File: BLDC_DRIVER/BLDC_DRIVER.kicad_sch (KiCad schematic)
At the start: 0 parts

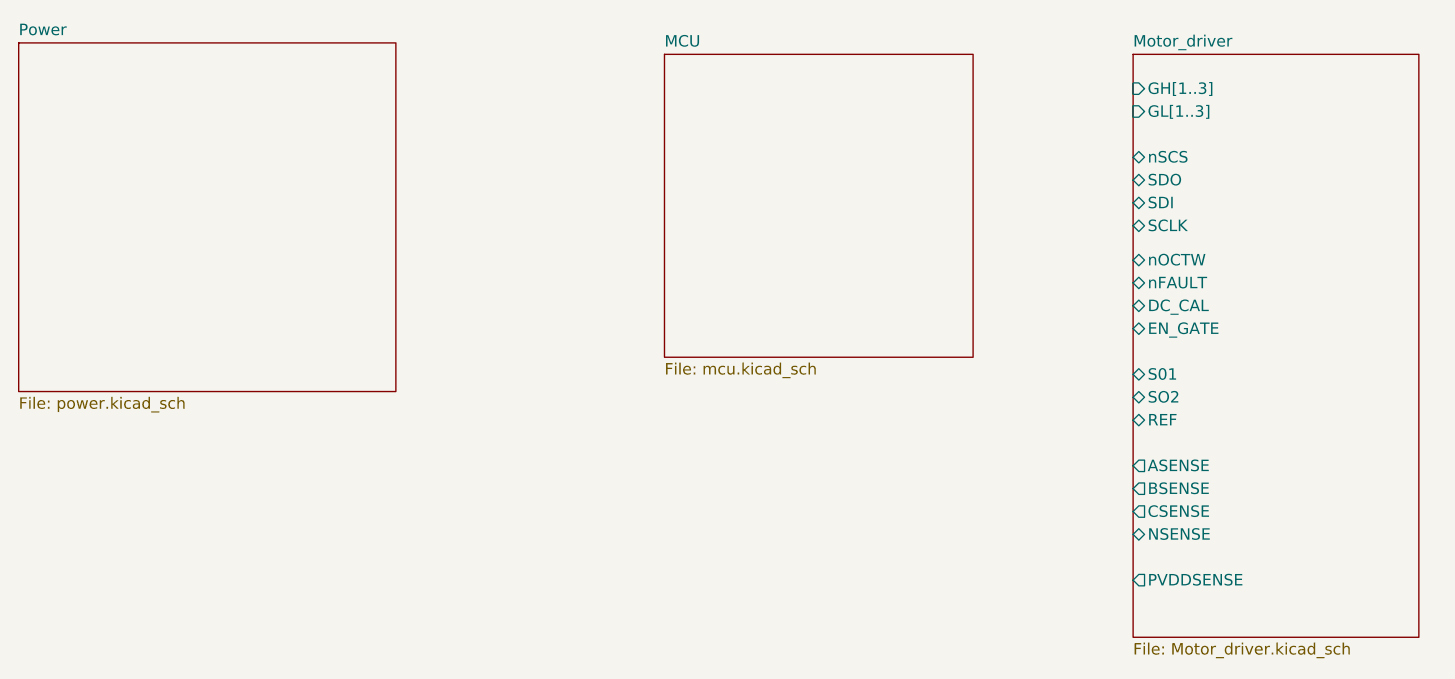
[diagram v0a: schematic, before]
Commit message: new driver
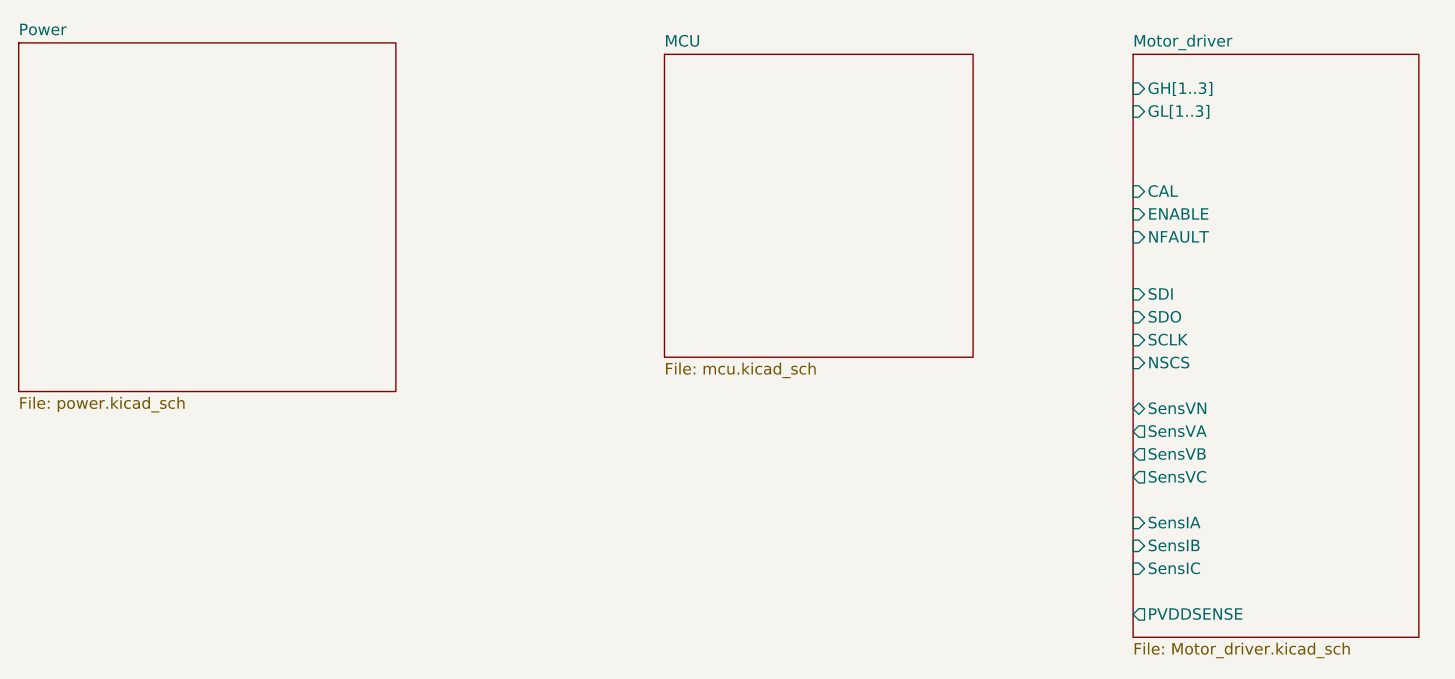
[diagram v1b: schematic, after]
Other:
- sheet Motor_driver ports: added CAL, ENABLE, NFAULT, NSCS, SensIA, SensIB, SensIC, SensVA, SensVB, SensVC, SensVN; removed ASENSE, BSENSE, CSENSE, DC_CAL, EN_GATE, NSENSE, REF, S01, SO2, nFAULT, nOCTW, nSCS
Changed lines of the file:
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@@
 			)
 		)
-		(pin "nFAULT" bidirectional
-			(at 157.48 62.23 180)
+		(pin "PVDDSENSE" output
+			(at 157.48 99.06 180)
 			(effects
 				(font
@@
 			)
 		)
-		(pin "SDO" bidirectional
-			(at 157.48 50.8 180)
+		(pin "SDO" input
+			(at 157.48 66.04 180)
 			(effects
 				(font
@@
 			)
 		)
-		(pin "REF" bidirectional
-			(at 157.48 77.47 180)
+		(pin "SCLK" input
+			(at 157.48 68.58 180)
 			(effects
 				(font
@@
 			)
 		)
-		(pin "nSCS" bidirectional
-			(at 157.48 48.26 180)
+		(pin "SensIA" input
+			(at 157.48 88.9 180)
 			(effects
 				(font
@@
 			)
 		)
-		(pin "nOCTW" bidirectional
-			(at 157.48 59.69 180)
+		(pin "ENABLE" input
+			(at 157.48 54.61 180)
 			(effects
 				(font
@@
 			)
 		)
-		(pin "SCLK" bidirectional
-			(at 157.48 55.88 180)
+		(pin "CAL" input
+			(at 157.48 52.07 180)
 			(effects
 				(font
@@
 			)
 		)
-		(pin "DC_CAL" bidirectional
-			(at 157.48 64.77 180)
+		(pin "SensVB" output
+			(at 157.48 81.28 180)
 			(effects
 				(font
@@
 			)
 		)
-		(pin "SDI" bidirectional
-			(at 157.48 53.34 180)
+		(pin "SensVC" output
+			(at 157.48 83.82 180)
 			(effects
 				(font
@@
 			)
 		)
-		(pin "EN_GATE" bidirectional
-			(at 157.48 67.31 180)
+		(pin "SensVA" output
+			(at 157.48 78.74 180)
 			(effects
 				(font
@@
 			)
 		)
-		(pin "BSENSE" output
-			(at 157.48 85.09 180)
+		(pin "SensVN" bidirectional
+			(at 157.48 76.2 180)
 			(effects
 				(font
@@
 			)
 		)
-		(pin "S01" bidirectional
-			(at 157.48 72.39 180)
+		(pin "NFAULT" input
+			(at 157.48 57.15 180)
 			(effects
 				(font
@@
 			)
 		)
-		(pin "ASENSE" output
-			(at 157.48 82.55 180)
+		(pin "SensIC" input
+			(at 157.48 93.98 180)
 			(effects
 				(font
@@
 			)
 		)
-		(pin "SO2" bidirectional
-			(at 157.48 74.93 180)
+		(pin "SensIB" input
+			(at 157.48 91.44 180)
 			(effects
 				(font
@@
 			)
 		)
-		(pin "CSENSE" output
-			(at 157.48 87.63 180)
+		(pin "NSCS" input
+			(at 157.48 71.12 180)
 			(effects
 				(font
@@
 			)
 		)
-		(pin "PVDDSENSE" output
-			(at 157.48 95.25 180)
+		(pin "SDI" input
+			(at 157.48 63.5 180)
 			(effects
 				(font
-					(size 1.27 1.27)
-				)
-				(justify left)
-			)
-		)
-		(pin "NSENSE" bidirectional
-			(at 157.48 90.17 180)
-			(effects
-				(font
